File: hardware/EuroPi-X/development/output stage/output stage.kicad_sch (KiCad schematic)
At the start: 27 parts, among them J1 Conn_01x06_Pin, J2 Conn_01x06_Pin, U1 TL074

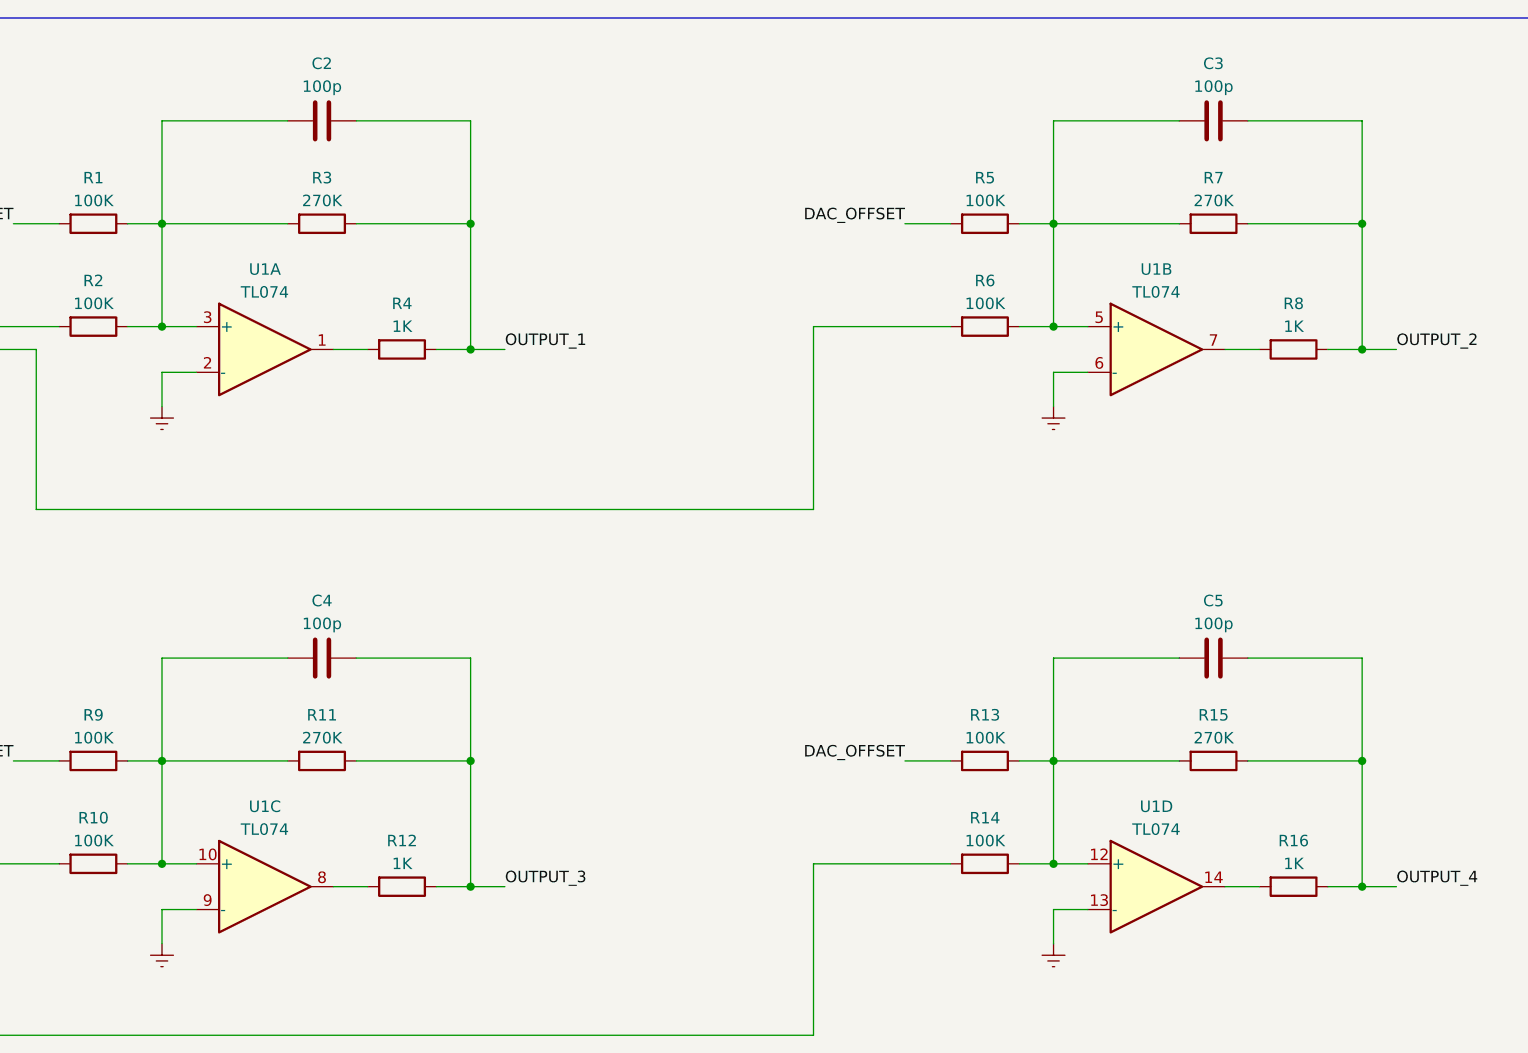
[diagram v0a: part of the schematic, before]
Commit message: save
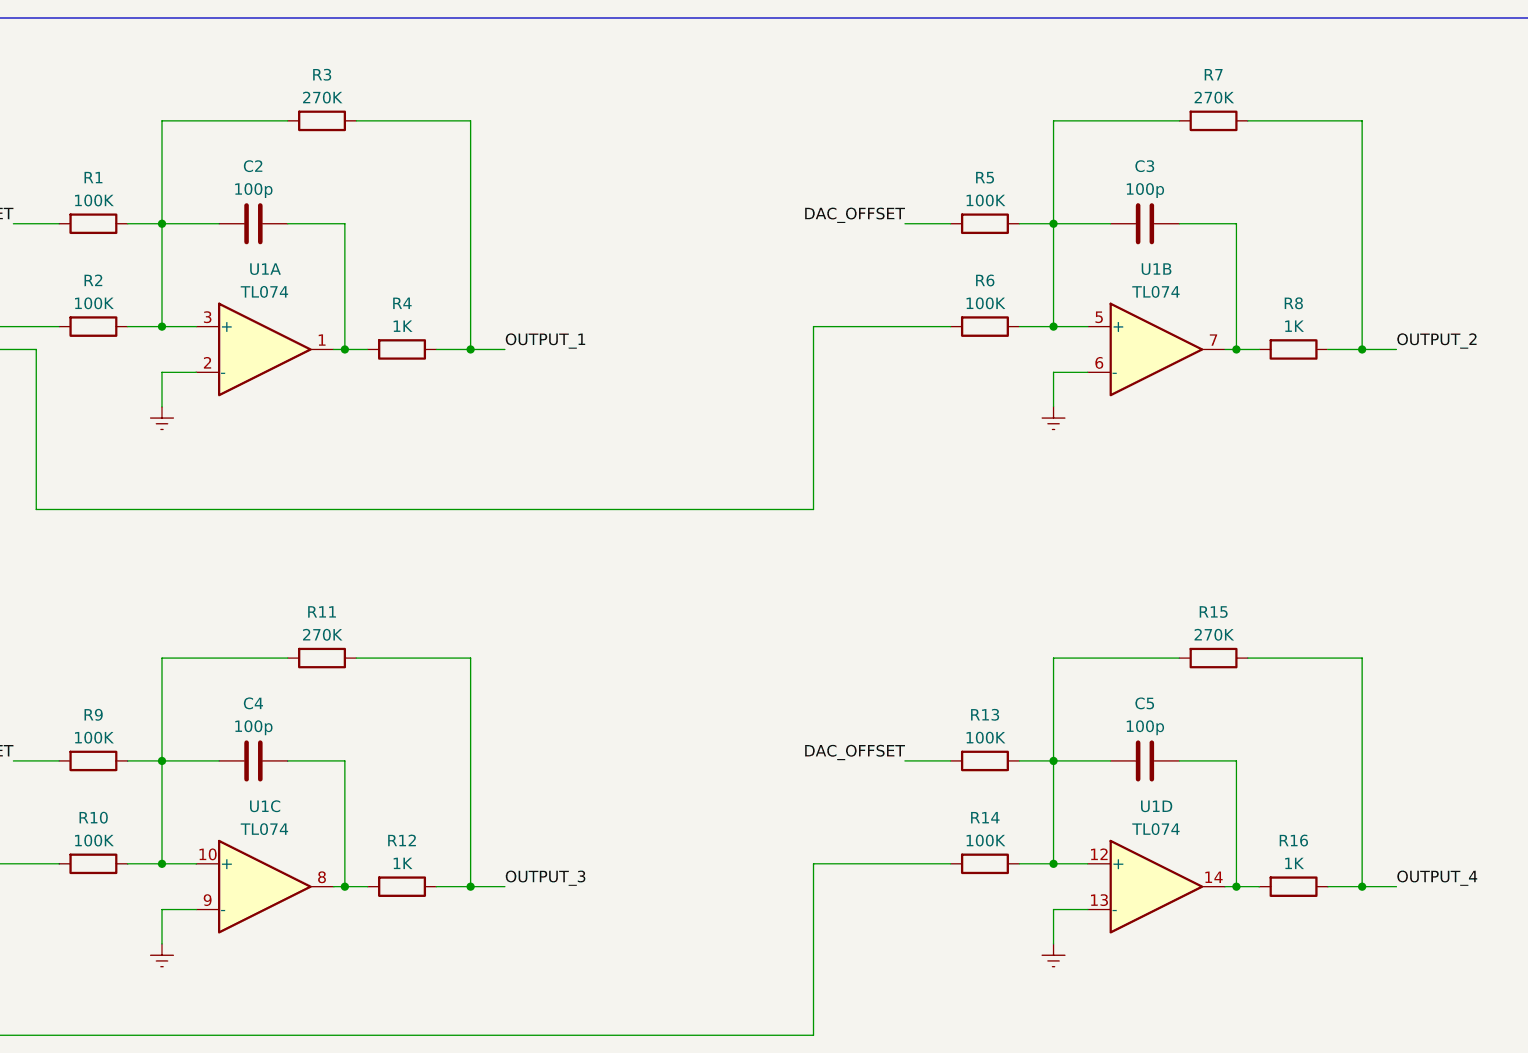
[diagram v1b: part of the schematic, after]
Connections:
- net OUTPUT_1: no longer C2.2
- net OUTPUT_2: no longer C3.2
- net OUTPUT_3: no longer C4.2
- net OUTPUT_4: no longer C5.2
- net at R4.2, U1.1: now also C2.2
- net at R8.2, U1.7: now also C3.2
- net at R16.2, U1.14: now also C5.2
- net at R12.2, U1.8: now also C4.2
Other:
- moved on the sheet: C2, C3, C4, C5, R11, R15, R3, R7
